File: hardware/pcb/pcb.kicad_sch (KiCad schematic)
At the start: 89 parts, among them K1 KEYSW, K10 KEYSW, K11 KEYSW, K12 KEYSW, K13 KEYSW, K14 KEYSW, K15 KEYSW, K16 KEYSW, K17 KEYSW, K18 KEYSW, K19 KEYSW, K2 KEYSW, K20 KEYSW, K21 KEYSW, K22 KEYSW, K23 KEYSW, K24 KEYSW, K25 KEYSW, K26 KEYSW, K27 KEYSW, K28 KEYSW, K29 KEYSW, K3 KEYSW, K30 KEYSW, K31 KEYSW, K32 KEYSW, K33 KEYSW, K34 KEYSW, K35 KEYSW, K36 KEYSW, K37 KEYSW, K38 KEYSW, K39 KEYSW, K4 KEYSW, K40 KEYSW, K41 KEYSW, K42 KEYSW, K43 KEYSW, K44 KEYSW, K5 KEYSW, K6 KEYSW, K7 KEYSW, K8 KEYSW, K9 KEYSW, U1 RP2040_Zero

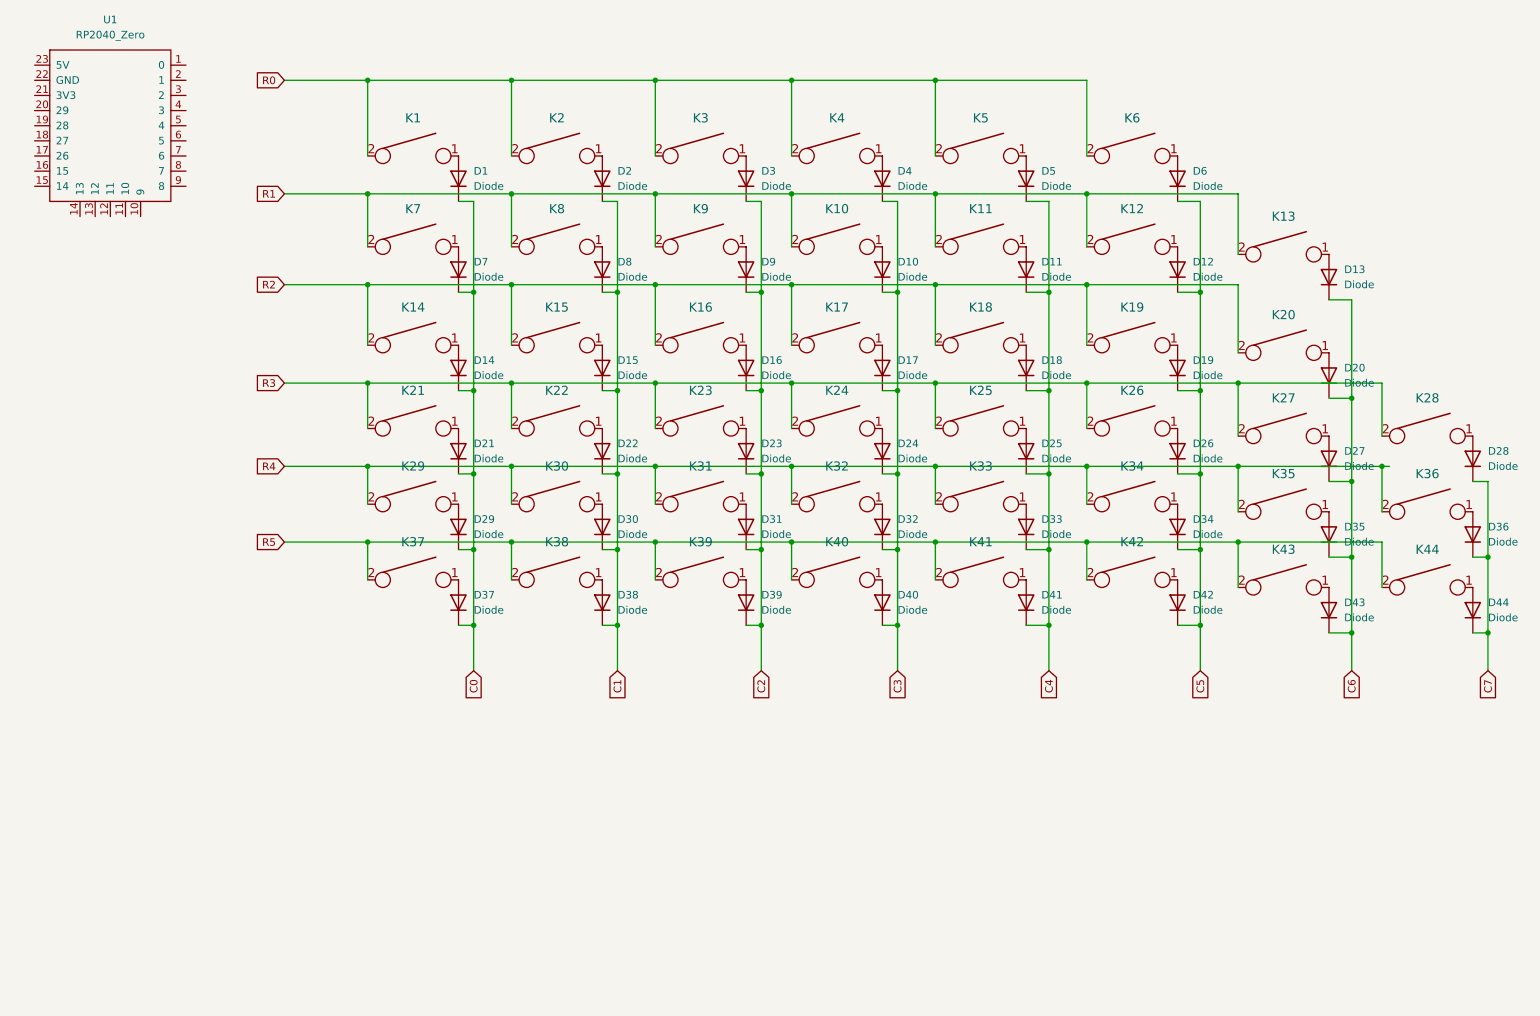
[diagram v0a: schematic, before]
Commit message: schema init
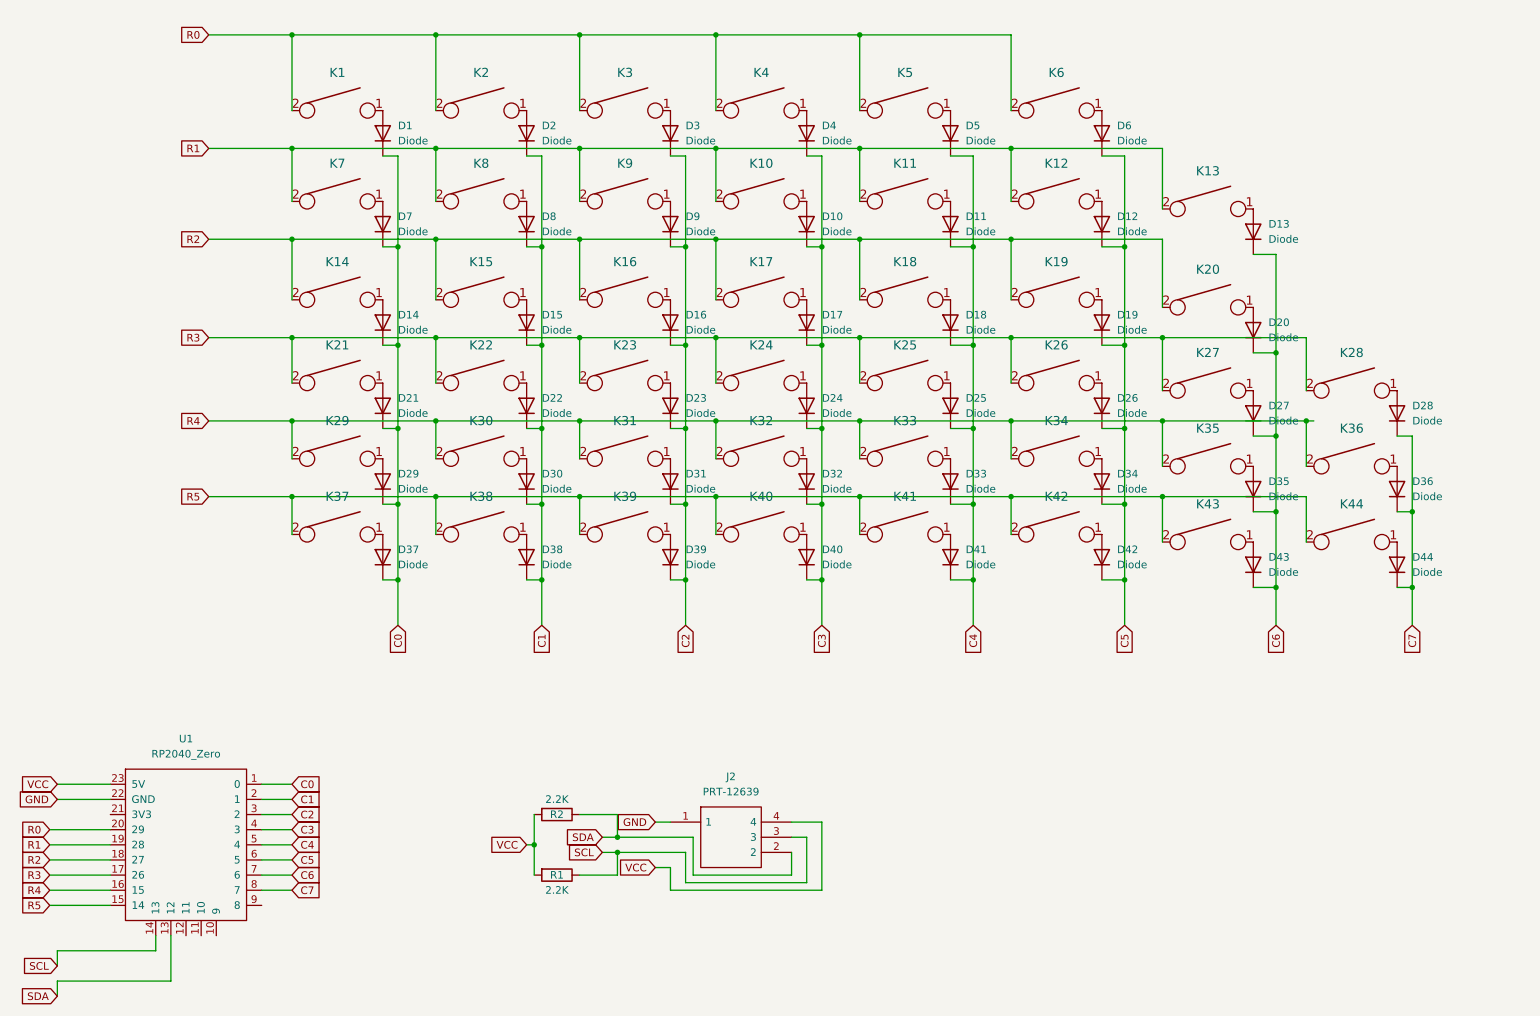
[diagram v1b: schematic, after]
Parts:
- added J2: PRT-12639, vbdox:PRT12639, symbol PRT-12639:PRT-12639
- added R1, R2: 2.2K, ScottoKeebs_Components:Diode_DO-35, symbol Device:R
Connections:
- net C0: now also U1.1 (0)
- net C1: now also U1.2 (1)
- net C2: now also U1.3 (2)
- net C3: now also U1.4 (3)
- net C4: now also U1.5 (4)
- net C5: now also U1.6 (5)
- net C6: now also U1.7 (6)
- net C7: now also U1.8 (7)
- net R0: now also U1.20 (29)
- net R1: now also U1.19 (28)
- net R2: now also U1.18 (27)
- net R3: now also U1.17 (26)
- net R4: now also U1.16 (15)
- net R5: now also U1.15 (14)
- net SDA: now reaches U1.13 (12)
- net SDA: now also J2.2, R2.1
- net SCL: now reaches U1.14 (13)
- net SCL: now also J2.3, R1.1
- net GND: now reaches U1.22 (GND)
- net GND: now also J2.1
- net VCC: now reaches U1.23 (5V)
- net VCC: now also J2.4, R1.2, R2.2
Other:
- moved on the sheet: D1, D10, D11, D12, D13, D14, D15, D16, D17, D18, D19, D2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
